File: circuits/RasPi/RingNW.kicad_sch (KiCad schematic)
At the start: 18 parts, among them J1 Conn_01x14_Pin, SW1 SW_SPST, U1 STM32F446RETx, Y1 16MHz

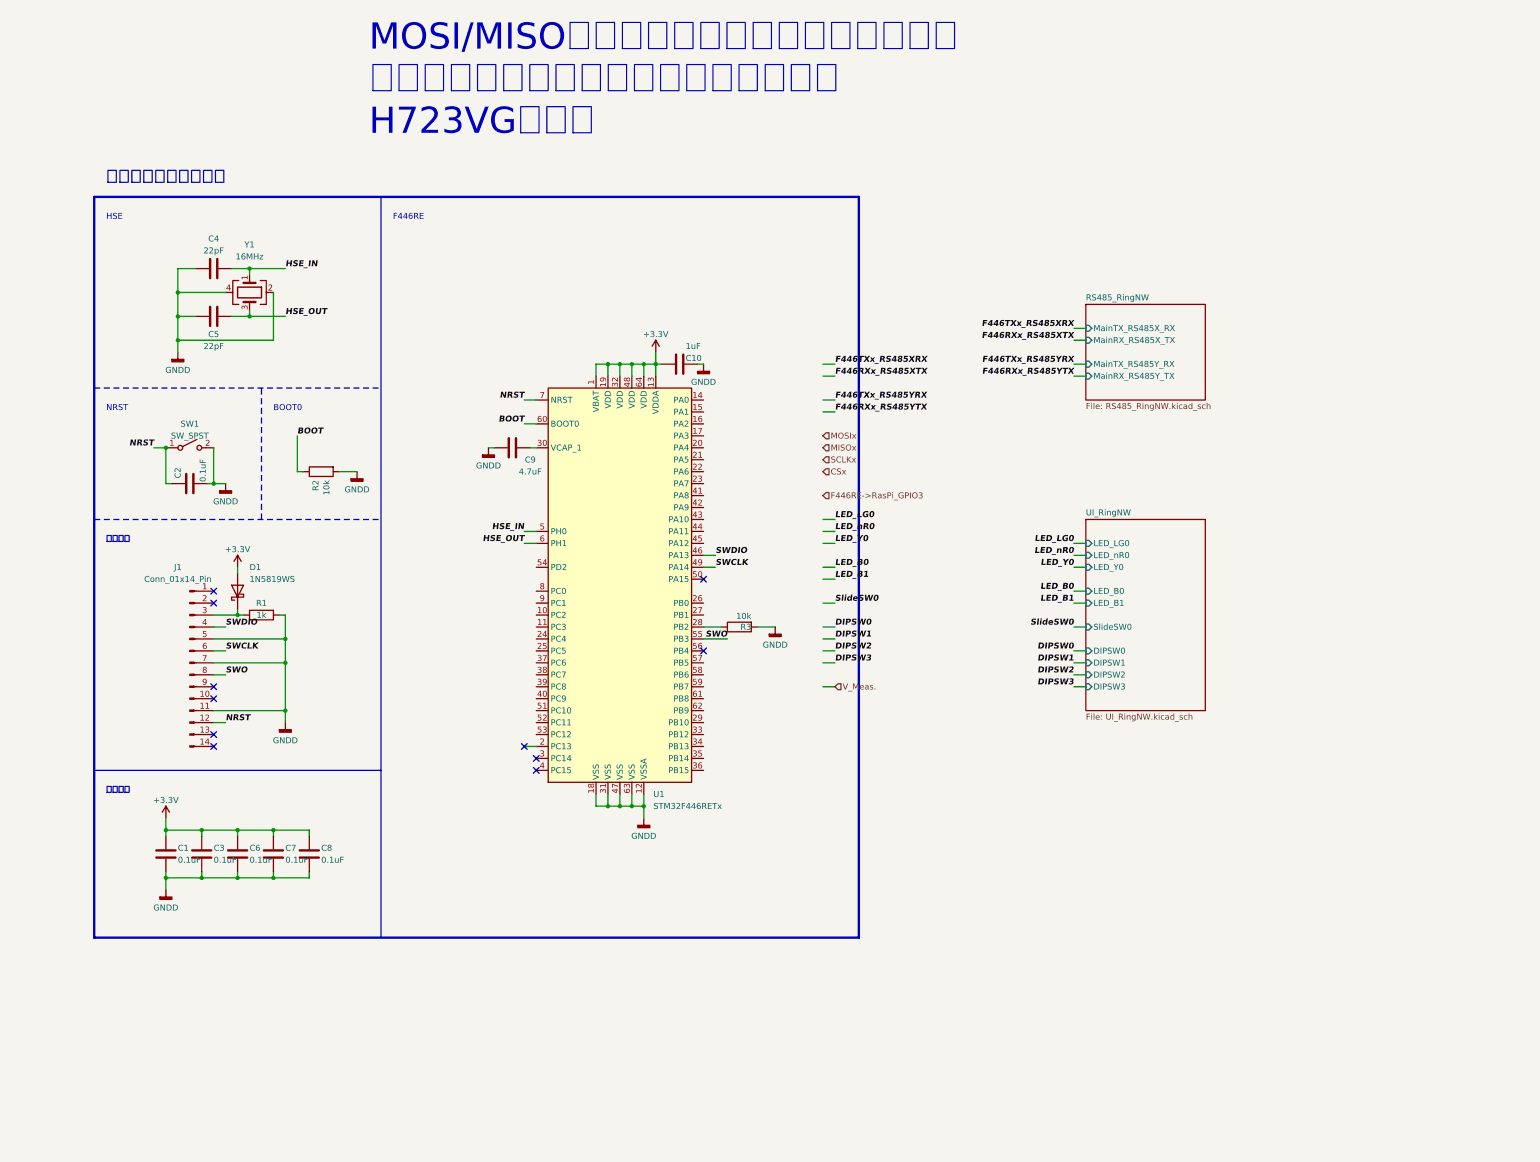
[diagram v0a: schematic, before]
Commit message: panelフットプリント配置
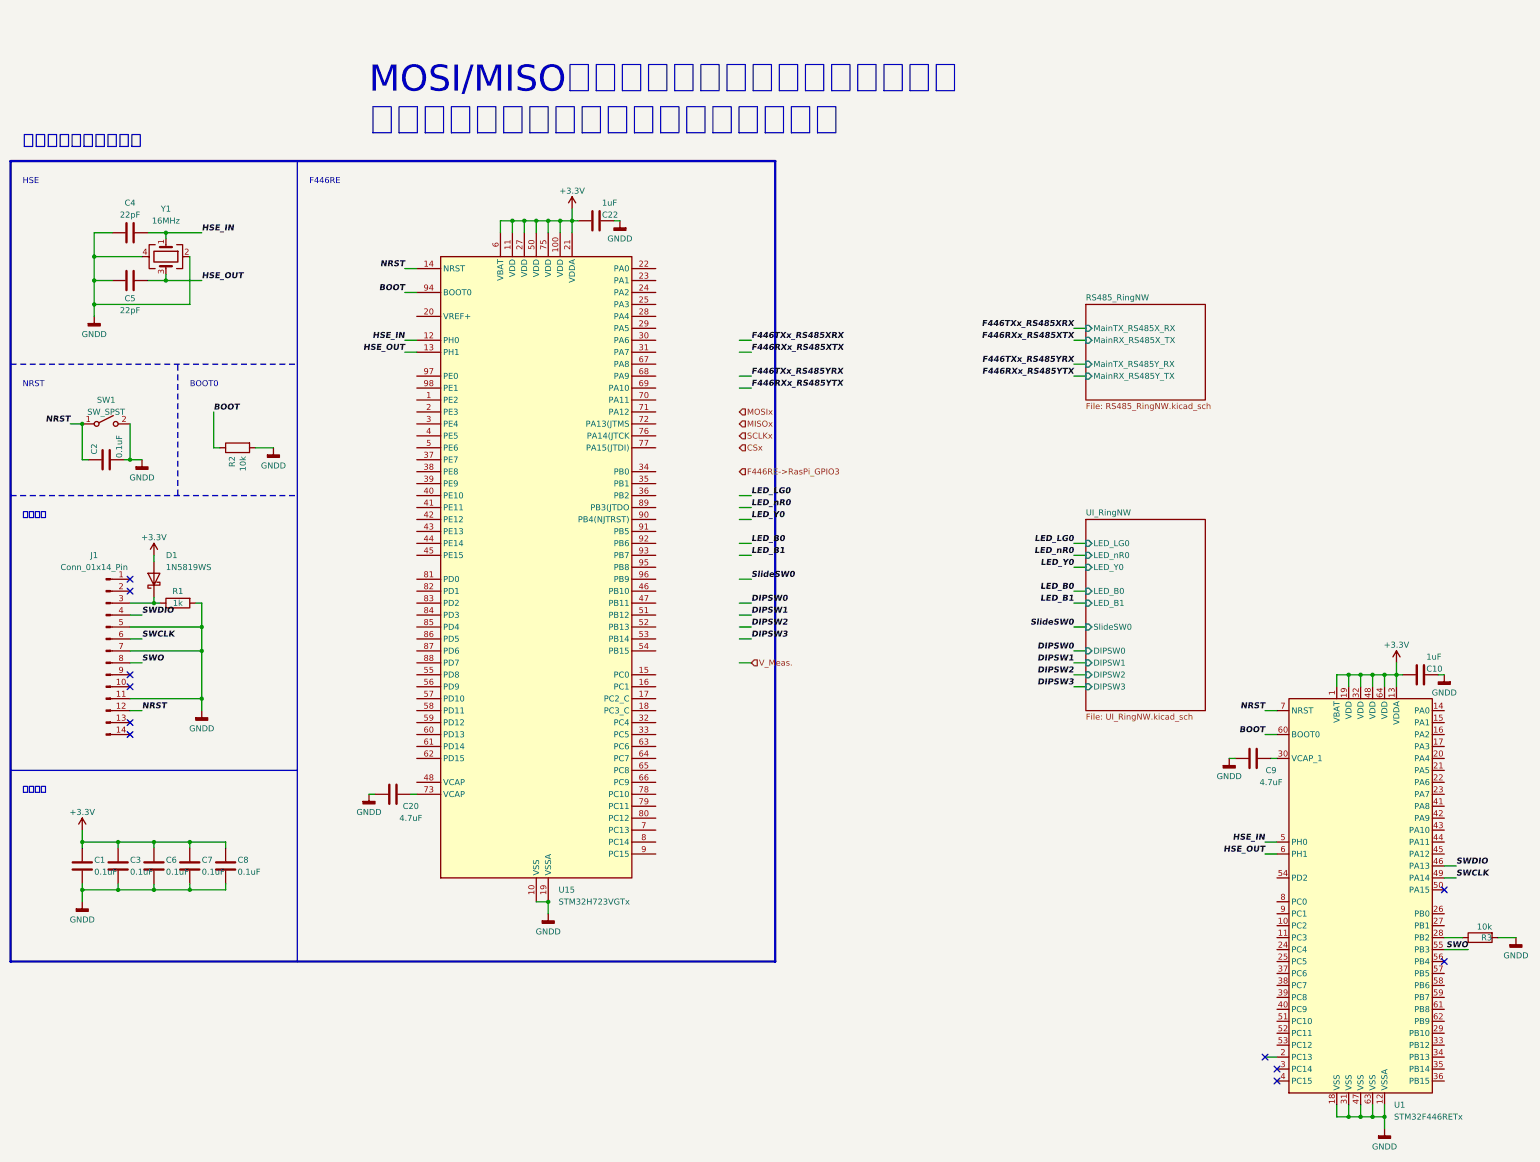
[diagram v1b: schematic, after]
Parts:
- added C20: 4.7uF, Capacitor_SMD:C_0603_1608Metric, symbol Device:C
- added C22: 1uF, Capacitor_SMD:C_0402_1005Metric, symbol Device:C
- added U15: STM32H723VGTx, Package_QFP:LQFP-100_14x14mm_P0.5mm, symbol MCU_ST_STM32H7:STM32H723VGTx
- U1: footprint Package_QFP:LQFP-64_10x10mm_P0.5mm -> (none)
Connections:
- net +3.3V: now also C22.2, U15.100 (VDD), U15.11 (VDD), U15.21 (VDDA), U15.27 (VDD), U15.50 (VDD), U15.6 (VBAT), U15.75 (VDD)
- net BOOT: now also U15.94 (BOOT0)
- net GNDD: now also C20.2, C22.1, U15.10 (VSS), U15.19 (VSSA), U15.26 (VSS), U15.49 (VSS), U15.74 (VSS), U15.99 (VSS)
- net HSE_IN: now also U15.12 (PH0)
- net HSE_OUT: now also U15.13 (PH1)
- net NRST: now also U15.14 (NRST)
- new net: C20.1, U15.73 (VCAP)
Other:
- note added: "MOSI/MISOはいつものとおんなじでいいのか いつもはマスターだけど今回はスレーブ"
- note removed: "MOSI/MISOはいつものとおんなじでいいのか いつもはマスターだけど今回はスレーブ H723VGにする"
- moved on the sheet: C1, C10, C2, C3, C4, C5, C6, C7, C8, C9, D1, J1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
